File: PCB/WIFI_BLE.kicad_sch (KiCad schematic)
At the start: 1 part, among them U8 LBEE5PK2AE-771

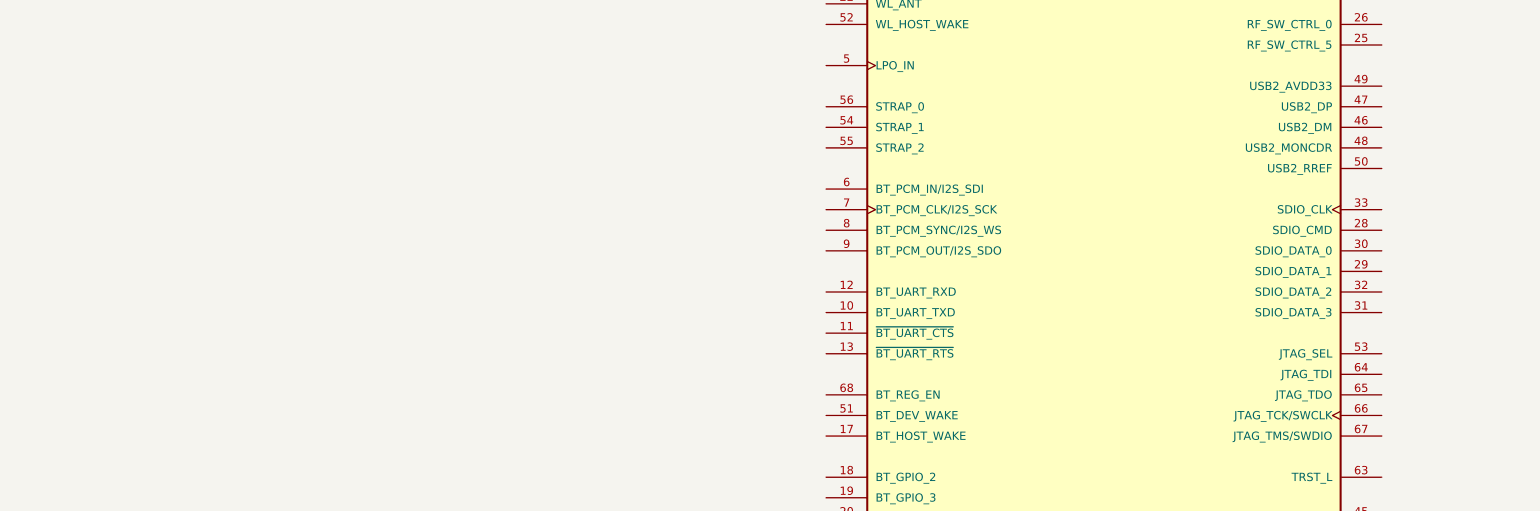
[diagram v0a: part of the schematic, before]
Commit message: PCB_UPDATE
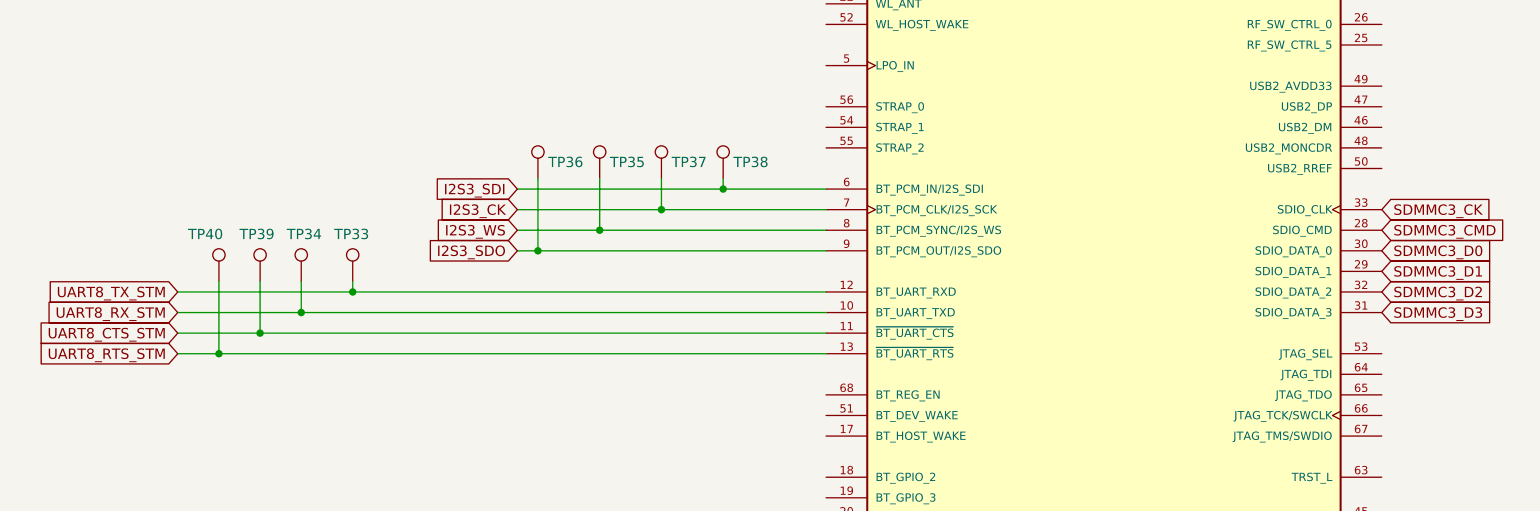
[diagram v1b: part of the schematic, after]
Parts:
- added TP33, TP34, TP35, TP36, TP37, TP38, TP39, TP40: TestPoint, TestPoint:TestPoint_Pad_D1.0mm, symbol Connector:TestPoint
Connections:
- net UART8_RX_STM: now reaches U8.10 (BT_UART_TXD)
- net UART8_RX_STM: now also TP34.1
- net UART8_CTS_STM: now reaches U8.11 (~{BT_UART_CTS})
- net UART8_CTS_STM: now also TP39.1
- net UART8_TX_STM: now reaches U8.12 (BT_UART_RXD)
- net UART8_TX_STM: now also TP33.1
- net UART8_RTS_STM: now reaches U8.13 (~{BT_UART_RTS})
- net UART8_RTS_STM: now also TP40.1
- net SDMMC3_CMD: now reaches U8.28 (SDIO_CMD)
- net SDMMC3_D1: now reaches U8.29 (SDIO_DATA_1)
- net SDMMC3_D0: now reaches U8.30 (SDIO_DATA_0)
- net SDMMC3_D3: now reaches U8.31 (SDIO_DATA_3)
- net SDMMC3_D2: now reaches U8.32 (SDIO_DATA_2)
- net SDMMC3_CK: now reaches U8.33 (SDIO_CLK)
- net I2S3_SDI: now reaches U8.6 (BT_PCM_IN/I2S_SDI)
- net I2S3_SDI: now also TP38.1
- net I2S3_CK: now reaches U8.7 (BT_PCM_CLK/I2S_SCK)
- net I2S3_CK: now also TP37.1
- net I2S3_WS: now reaches U8.8 (BT_PCM_SYNC/I2S_WS)
- net I2S3_WS: now also TP35.1
- net I2S3_SDO: now reaches U8.9 (BT_PCM_OUT/I2S_SDO)
- net I2S3_SDO: now also TP36.1

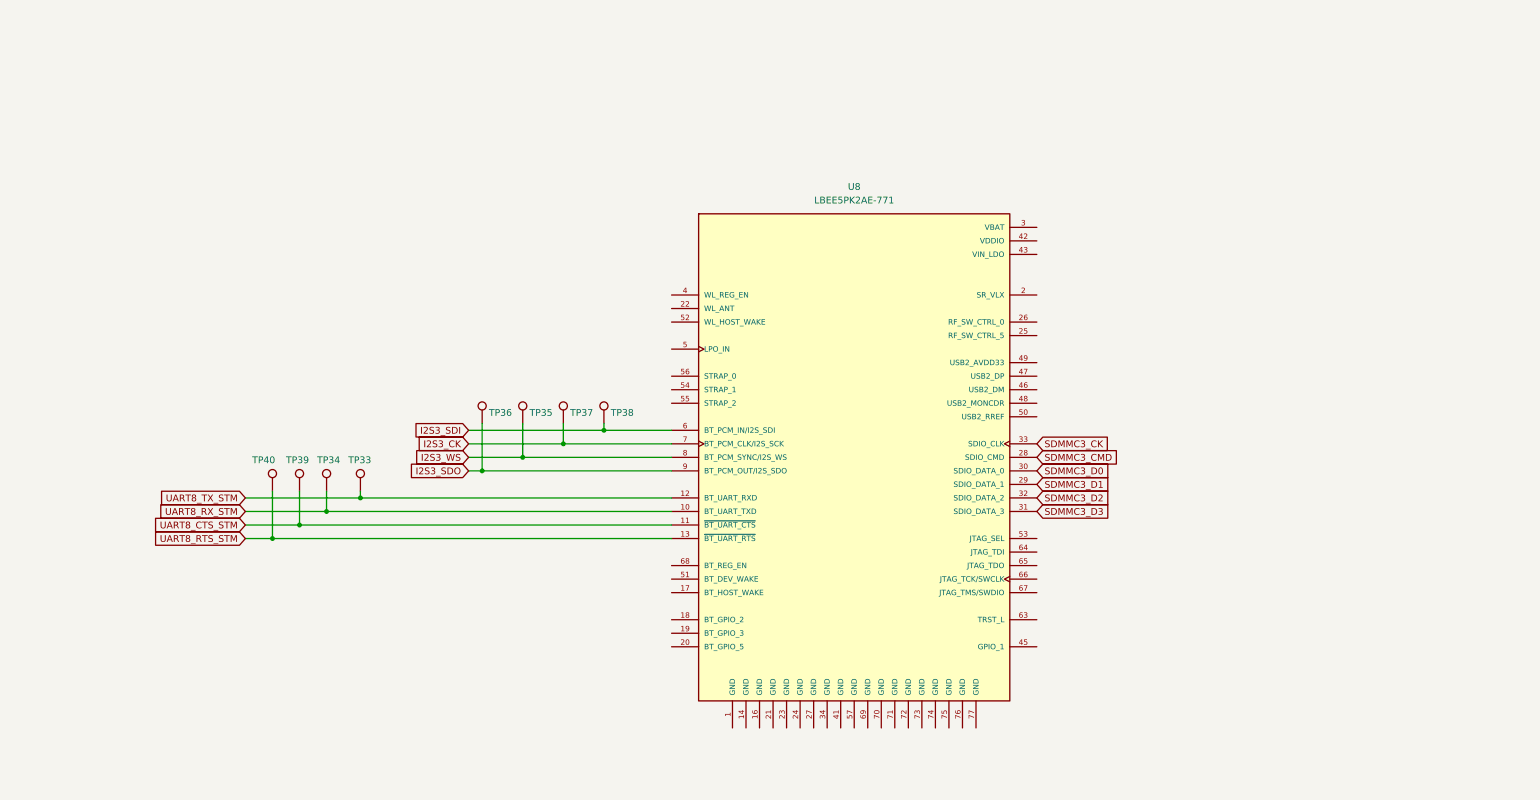
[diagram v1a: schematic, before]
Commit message: wifi done
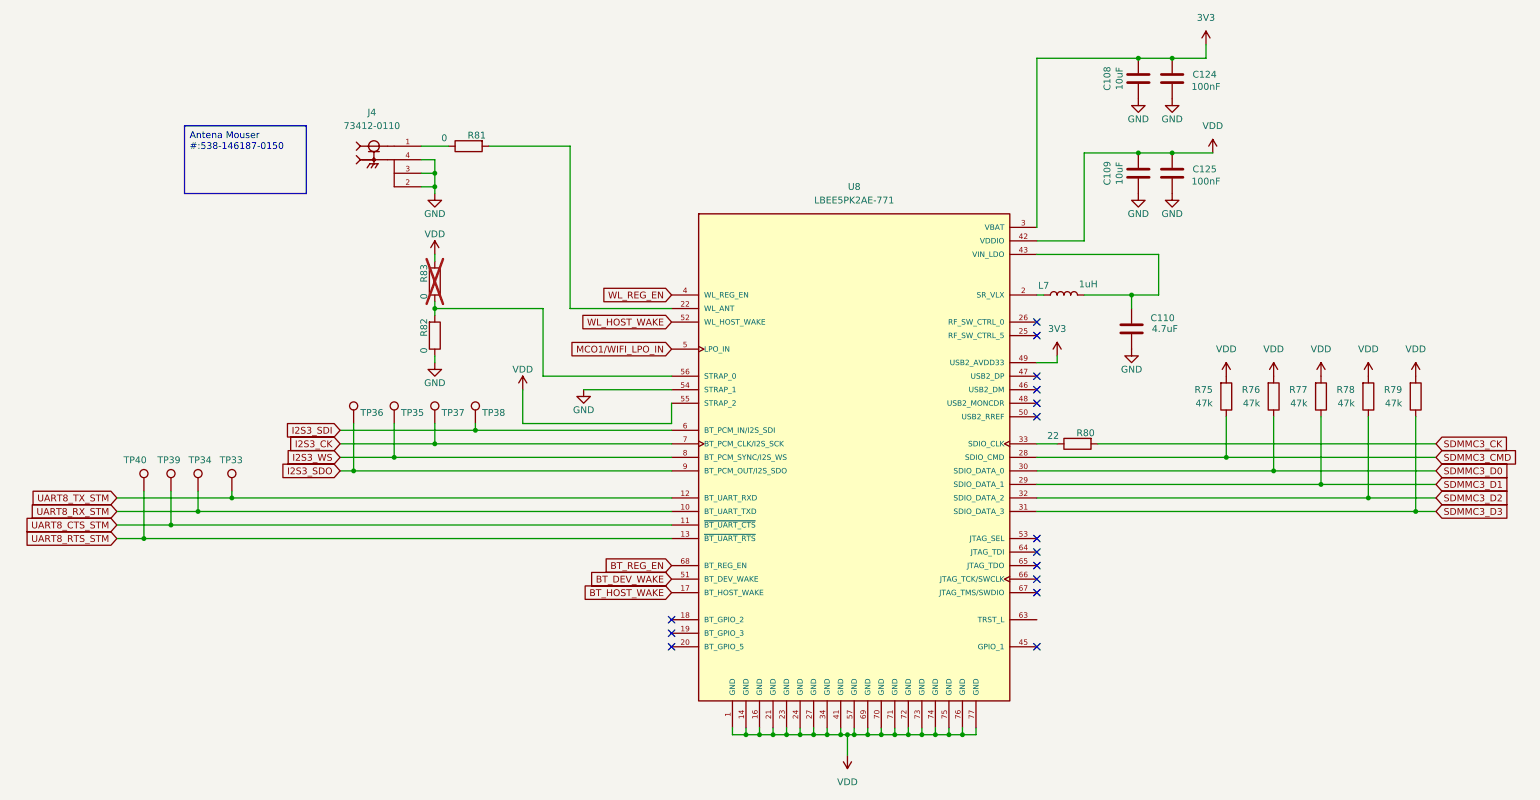
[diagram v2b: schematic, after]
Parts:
- added C108, C109: 10uF, Capacitor_SMD:C_0603_1608Metric, symbol Device:C
- added C110: 4.7uF, Capacitor_SMD:C_0402_1005Metric, symbol Device:C
- added C124, C125: 100nF, Capacitor_SMD:C_0402_1005Metric, symbol Device:C
- added J4: 73412-0110, 73412-0110:MOLEX_73412-0110, symbol 73412-0110:73412-0110
- added L7: 1uH, Inductor_SMD:L_Murata_DFE201610P, symbol Device:L
- added R75, R76, R77, R78, R79: 47k, Resistor_SMD:R_0402_1005Metric, symbol Device:R
- added R80: 22, Resistor_SMD:R_0402_1005Metric, symbol Device:R
- added R81, R82, R83: 0, Resistor_SMD:R_0402_1005Metric, symbol Device:R
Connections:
- net SDMMC3_CK: now also R80.2; no longer U8.33 (SDIO_CLK)
- net SDMMC3_CMD: now also R75.1
- net SDMMC3_D0: now also R76.1
- net SDMMC3_D1: now also R77.1
- net SDMMC3_D2: now also R78.1
- net SDMMC3_D3: now also R79.1
- net VDD: now reaches U8.1 (GND)
- net VDD: now also U8.14 (GND), U8.16 (GND), U8.21 (GND), U8.23 (GND), U8.24 (GND), U8.27 (GND), U8.34 (GND), U8.41 (GND), U8.42 (VDDIO), U8.55 (STRAP_2), U8.57 (GND), U8.69 (GND), U8.70 (GND), U8.71 (GND), U8.72 (GND), U8.73 (GND), U8.74 (GND), U8.75 (GND), U8.76 (GND), U8.77 (GND), C109.2, C125.2, R75.2, R76.2, R77.2, R78.2, R79.2, R83.2
- net BT_HOST_WAKE: now reaches U8.17 (BT_HOST_WAKE)
- net at U8.2 (SR_VLX): now also L7.1
- net at U8.22 (WL_ANT): now also R81.2
- net 3V3: now reaches U8.3 (VBAT)
- net 3V3: now also U8.49 (USB2_AVDD33), C108.2, C124.2
- net WL_REG_EN: now reaches U8.4 (WL_REG_EN)
- net at U8.43 (VIN_LDO): now also C110.2, L7.2
- net MCO1/WIFI_LPO_IN: now reaches U8.5 (LPO_IN)
- net BT_DEV_WAKE: now reaches U8.51 (BT_DEV_WAKE)
- net WL_HOST_WAKE: now reaches U8.52 (WL_HOST_WAKE)
- net GND: now reaches U8.54 (STRAP_1)
- net GND: now also C108.1, C109.1, C110.1, C124.1, C125.1, J4.2, J4.3, J4.4, R82.1
- net at U8.56 (STRAP_0): now also R82.2, R83.1
- net BT_REG_EN: now reaches U8.68 (BT_REG_EN)
- new net: R80.1, U8.33 (SDIO_CLK)
- new net: J4.1, R81.1
- no-connect marks 0 -> 15
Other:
- moved on the sheet: TP33, TP34, TP35, TP36, TP37, TP38, TP39, TP40
